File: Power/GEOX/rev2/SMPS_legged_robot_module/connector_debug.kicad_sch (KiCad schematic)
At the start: 7 parts, among them J601 98414-G06-12ULF, U601 24LC025-I/ST

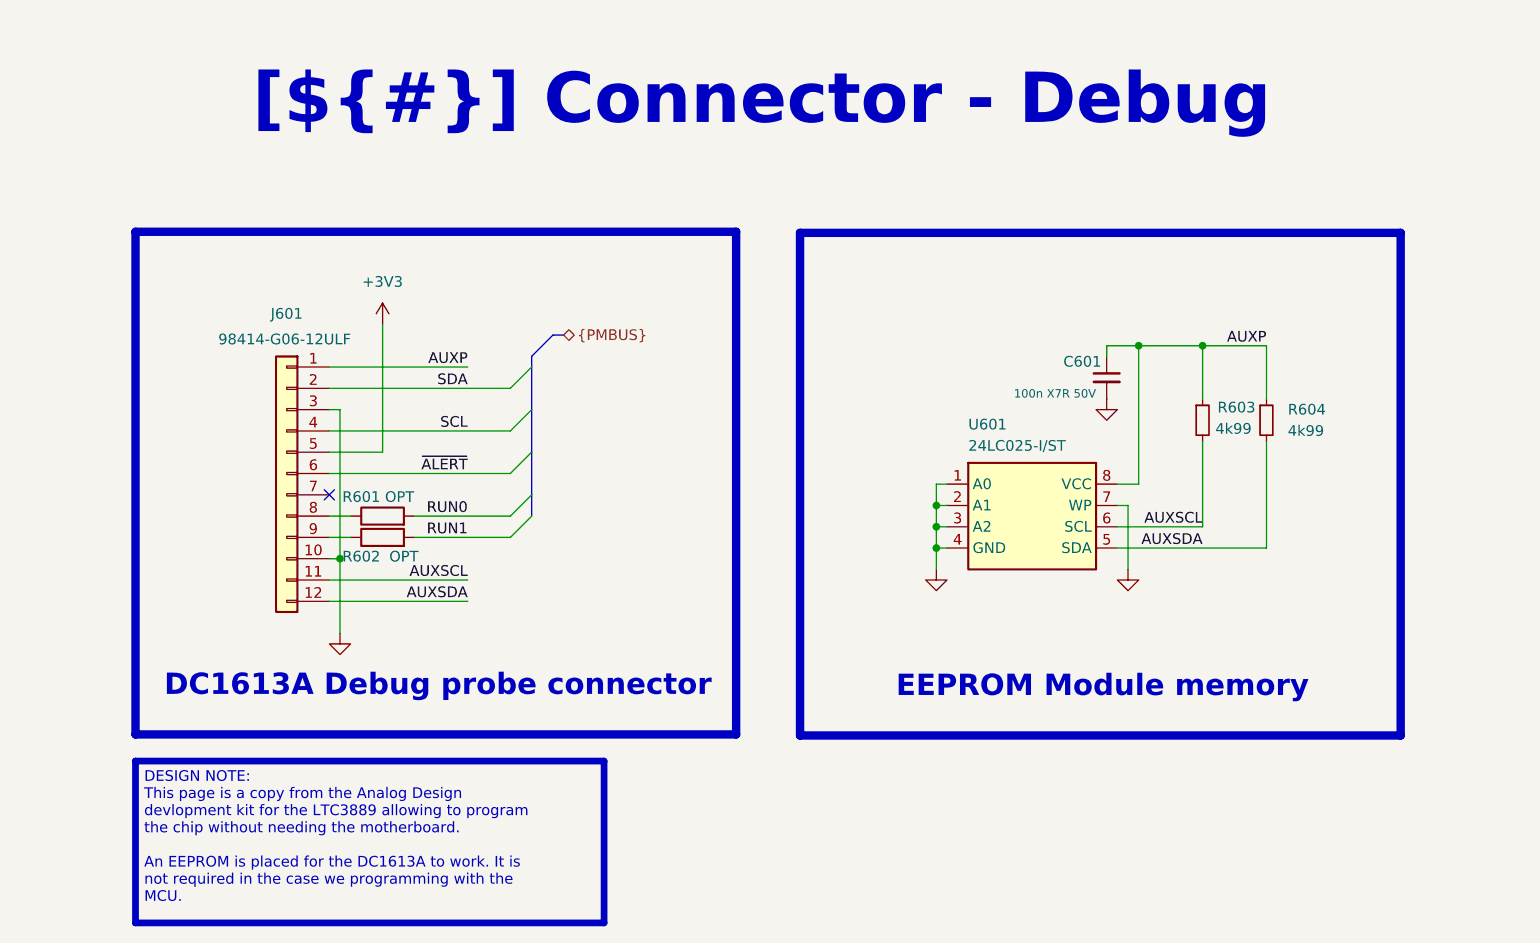
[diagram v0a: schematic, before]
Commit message: Nothing to declare
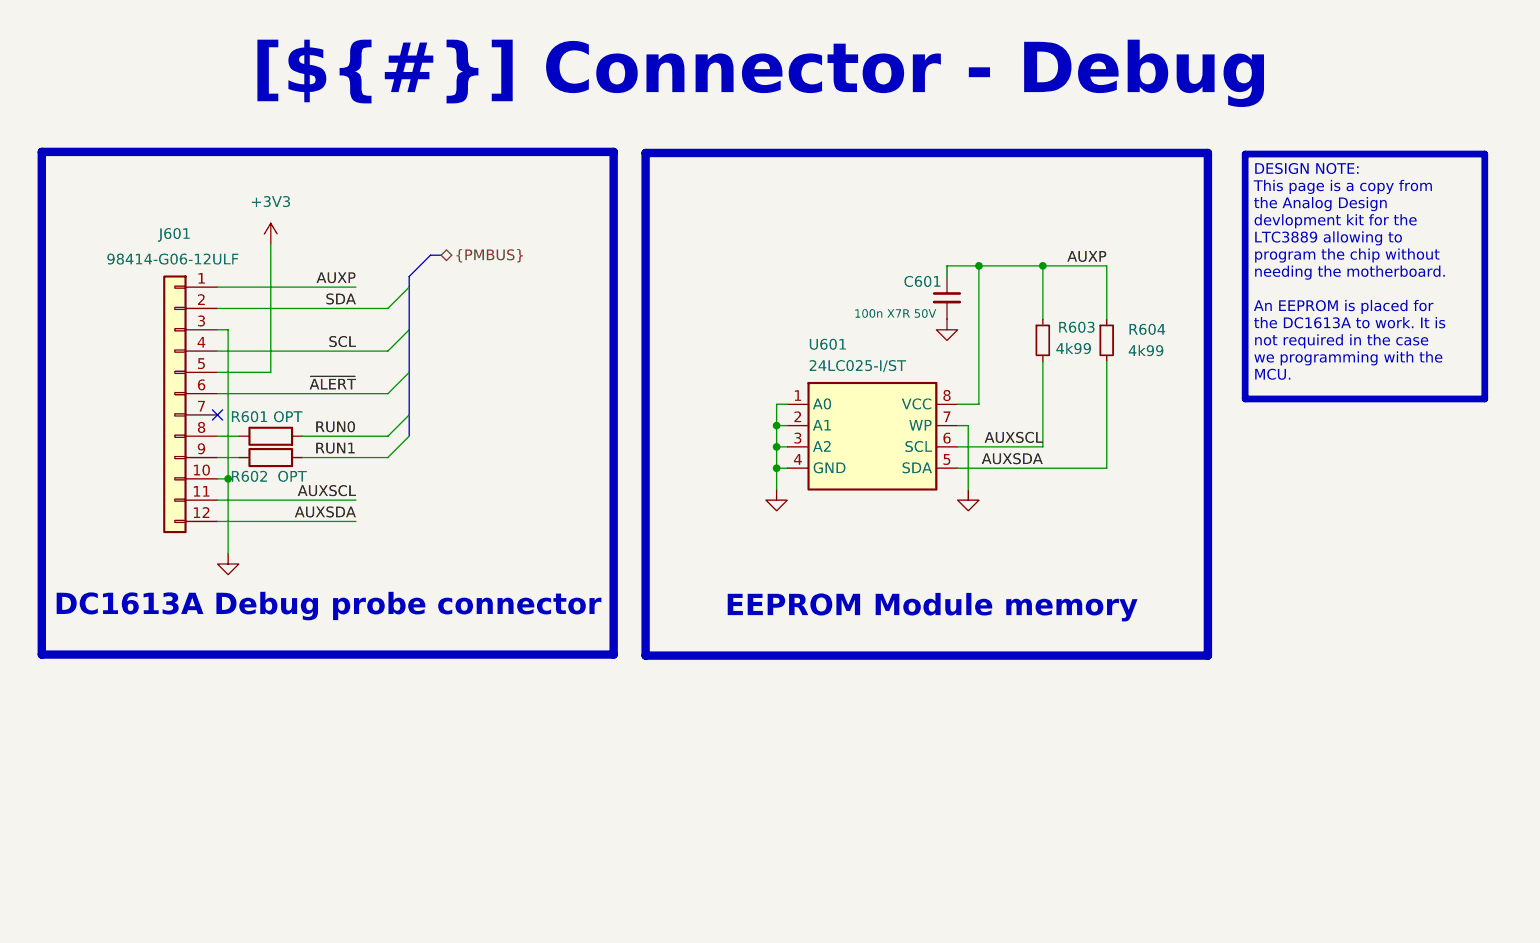
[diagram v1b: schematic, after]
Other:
- moved on the sheet: C601, J601, R601, R602, R603, R604, U601
